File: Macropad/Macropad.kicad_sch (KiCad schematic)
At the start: 66 parts, among them J1 TSOP4838_C124647, J2 IR_LED_TX_HDR, J3 LED_CHAIN, J4 LCD_SPI_PWRDATA, J5 LCD_SPI_CTRL, J6 TOUCH_I2C_SD_IRQ, J7 BATTERY_LIPO, J8 BAT_PMIC_IO, SW1 SW_Push, SW10 SW_Push, SW11 SW_Push, SW12 SW_Push, SW13 SW_Push, SW14 SW_Push, SW15 SW_Push, SW16 SW_Push, SW17 SW_Push, SW18 SW_Push, SW19 SW_Push, SW2 SW_Push, SW20 SW_Push, SW21 SW_Push, SW22 SW_Push, SW23 SW_Push, SW24 SW_Push, SW25 SW_Push, SW26 SW_Push, SW27 RotaryEncoder_Switch, SW3 SW_Push, SW4 SW_Push, SW5 SW_Push, SW6 SW_Push, SW7 SW_Push, SW8 SW_Push, SW9 SW_Push, U901A1 ESP32S3_WROOM1_LEFT, U901B1 ESP32S3_WROOM1_RIGHT

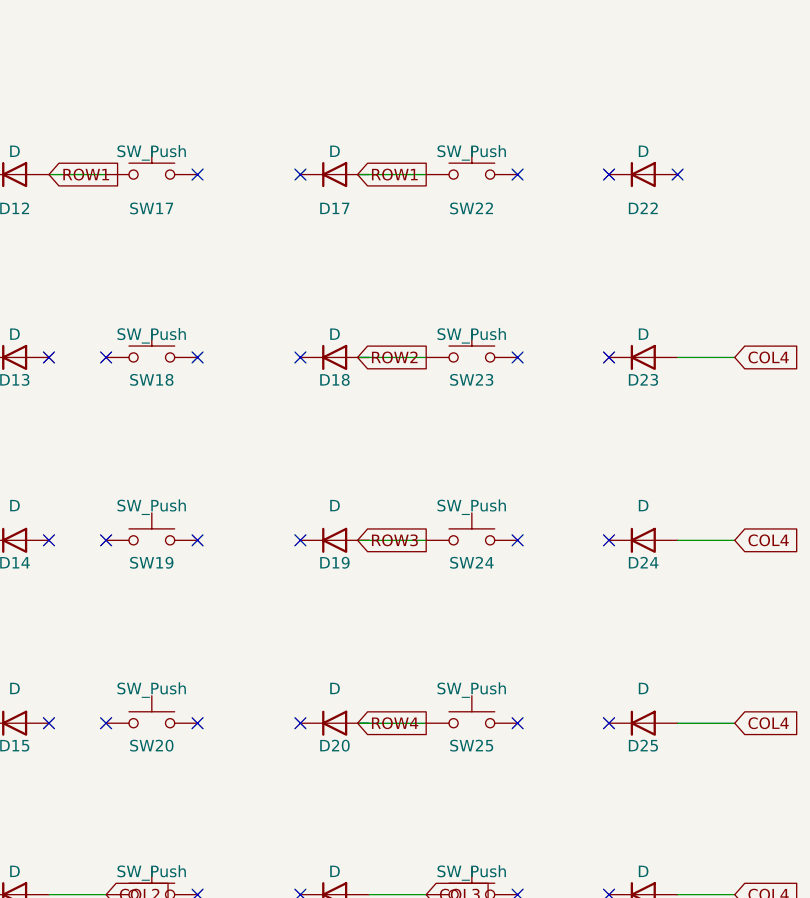
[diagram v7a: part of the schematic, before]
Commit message: Updates
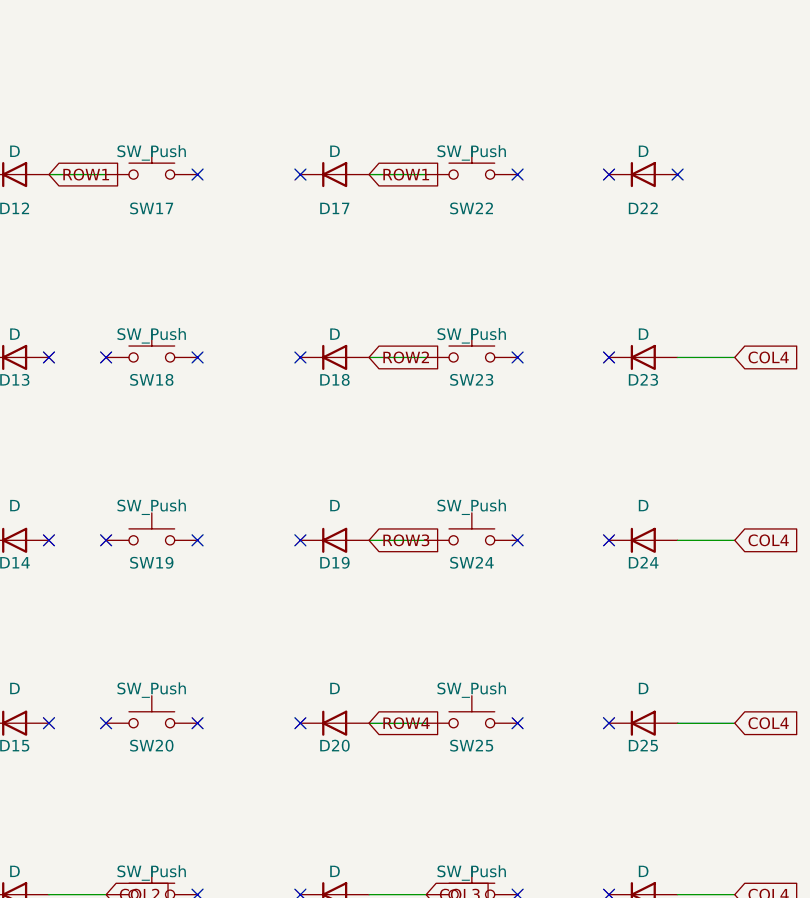
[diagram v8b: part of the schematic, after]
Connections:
- net ROW1: now also D17.2 (A)
- net ROW2: now also D18.2 (A)
- net ROW3: now also D19.2 (A)
- net ROW4: now also D20.2 (A)
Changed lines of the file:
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@@
 	(wire
 		(pts
-			(xy 167.64 74.93) (xy 175.26 74.93)
+			(xy 168.91 74.93) (xy 175.26 74.93)
 		)
 		(stroke
@@
 	(wire
 		(pts
-			(xy 167.64 95.25) (xy 175.26 95.25)
+			(xy 168.91 95.25) (xy 175.26 95.25)
 		)
 		(stroke
@@
 	(wire
 		(pts
-			(xy 167.64 54.61) (xy 175.26 54.61)
+			(xy 168.91 54.61) (xy 175.26 54.61)
 		)
 		(stroke
@@
 	(wire
 		(pts
-			(xy 167.64 115.57) (xy 175.26 115.57)
+			(xy 168.91 115.57) (xy 175.26 115.57)
 		)
 		(stroke
@@
 	(global_label "ROW1"
 		(shape input)
-		(at 167.64 54.61 0)
-		(fields_autoplaced yes)
-		(effects
-			(font
-				(size 1.27 1.27)
-				(thickness 0.15)
-			)
-		)
-		(property "Intersheetrefs" "${INTERSHEET_REFS}"
-			(at 167.64 54.61 0)
+		(at 168.91 54.61 0)
+		(fields_autoplaced yes)
+		(effects
+			(font
+				(size 1.27 1.27)
+				(thickness 0.15)
+			)
+		)
+		(property "Intersheetrefs" "${INTERSHEET_REFS}"
+			(at 168.91 54.61 0)
 			(effects
 				(font
@@
 	(global_label "ROW4"
 		(shape input)
-		(at 167.64 115.57 0)
-		(fields_autoplaced yes)
-		(effects
-			(font
-				(size 1.27 1.27)
-				(thickness 0.15)
-			)
-		)
-		(property "Intersheetrefs" "${INTERSHEET_REFS}"
-			(at 167.64 115.57 0)
+		(at 168.91 115.57 0)
+		(fields_autoplaced yes)
+		(effects
+			(font
+				(size 1.27 1.27)
+				(thickness 0.15)
+			)
+		)
+		(property "Intersheetrefs" "${INTERSHEET_REFS}"
+			(at 168.91 115.57 0)
 			(effects
 				(font
@@
 	(global_label "ROW3"
 		(shape input)
-		(at 167.64 95.25 0)
-		(fields_autoplaced yes)
-		(effects
-			(font
-				(size 1.27 1.27)
-				(thickness 0.15)
-			)
-		)
-		(property "Intersheetrefs" "${INTERSHEET_REFS}"
-			(at 167.64 95.25 0)
+		(at 168.91 95.25 0)
+		(fields_autoplaced yes)
+		(effects
+			(font
+				(size 1.27 1.27)
+				(thickness 0.15)
+			)
+		)
+		(property "Intersheetrefs" "${INTERSHEET_REFS}"
+			(at 168.91 95.25 0)
 			(effects
 				(font
@@
 	(global_label "ROW2"
 		(shape input)
-		(at 167.64 74.93 0)
-		(fields_autoplaced yes)
-		(effects
-			(font
-				(size 1.27 1.27)
-				(thickness 0.15)
-			)
-		)
-		(property "Intersheetrefs" "${INTERSHEET_REFS}"
-			(at 167.64 74.93 0)
-			(effects
-				(font
+		(at 168.91 74.93 0)
+		(fields_autoplaced yes)
+		(effects
+			(font
+				(size 1.27 1.27)
+				(thickness 0.15)
+			)
+		)
+		(property "Intersheetrefs" "${INTERSHEET_REFS}"
+			(at 168.91 74.93 0)
+			(effects
+				(font
